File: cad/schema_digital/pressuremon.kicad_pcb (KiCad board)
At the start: 2 copper layers, 50 x 50 mm, 15 parts, among them J1 Conn_01x04_Pin, J2 Conn_01x04_Pin, J3 Force Config, SW1 SW_SPDT, U3 DS18B20

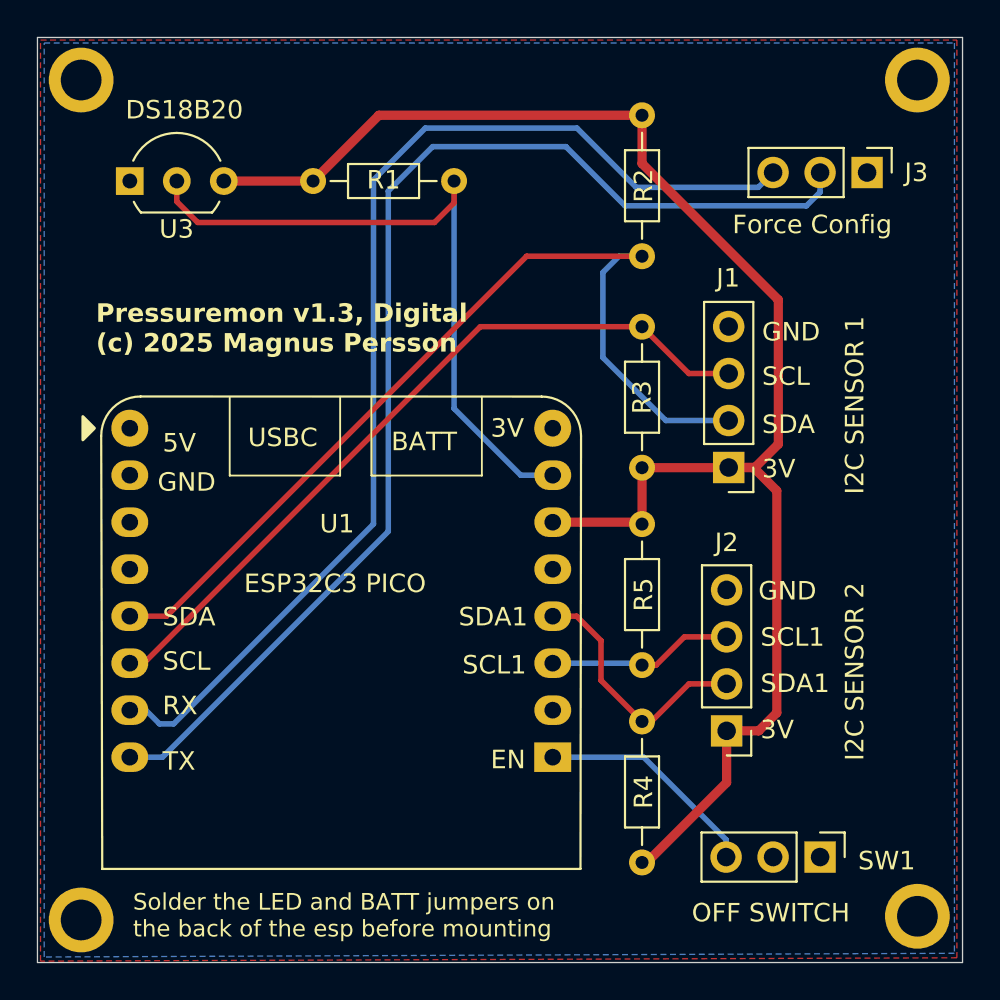
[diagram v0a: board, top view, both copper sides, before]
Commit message: Update analog pcb
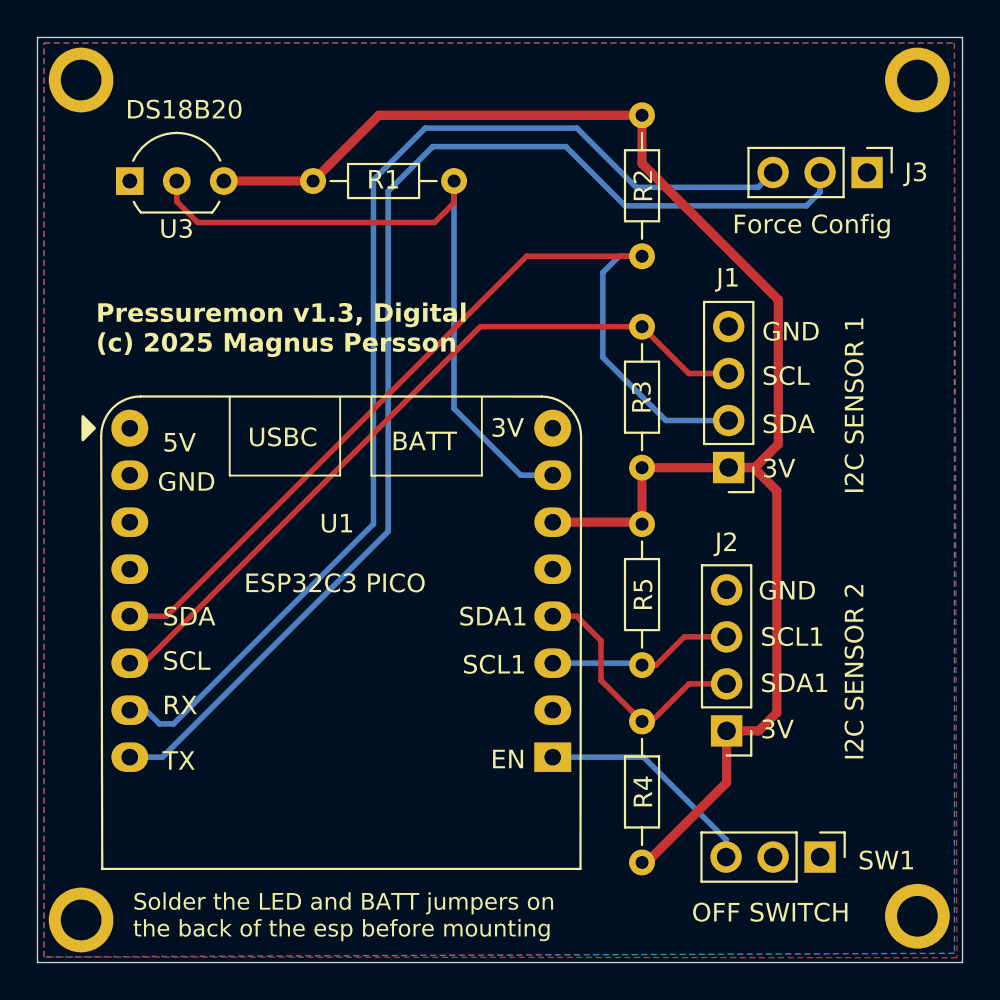
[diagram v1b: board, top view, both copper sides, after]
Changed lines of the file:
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@@
 		(polygon
 			(pts
-				(xy 108.204 40.64) (xy 157.734 40.64) (xy 157.734 90.243234) (xy 108.204 90.424)
+				(xy 108.4 40.8) (xy 157.6 40.8) (xy 157.734 90.243234) (xy 108.4 90.2)
 			)
 		)
